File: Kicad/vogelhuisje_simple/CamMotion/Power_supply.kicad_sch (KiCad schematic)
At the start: 11 parts, among them P1 TP4056breakout, P3 TP4056breakout, P4 TP4056breakout, Q1 Q_PMOS_DGS

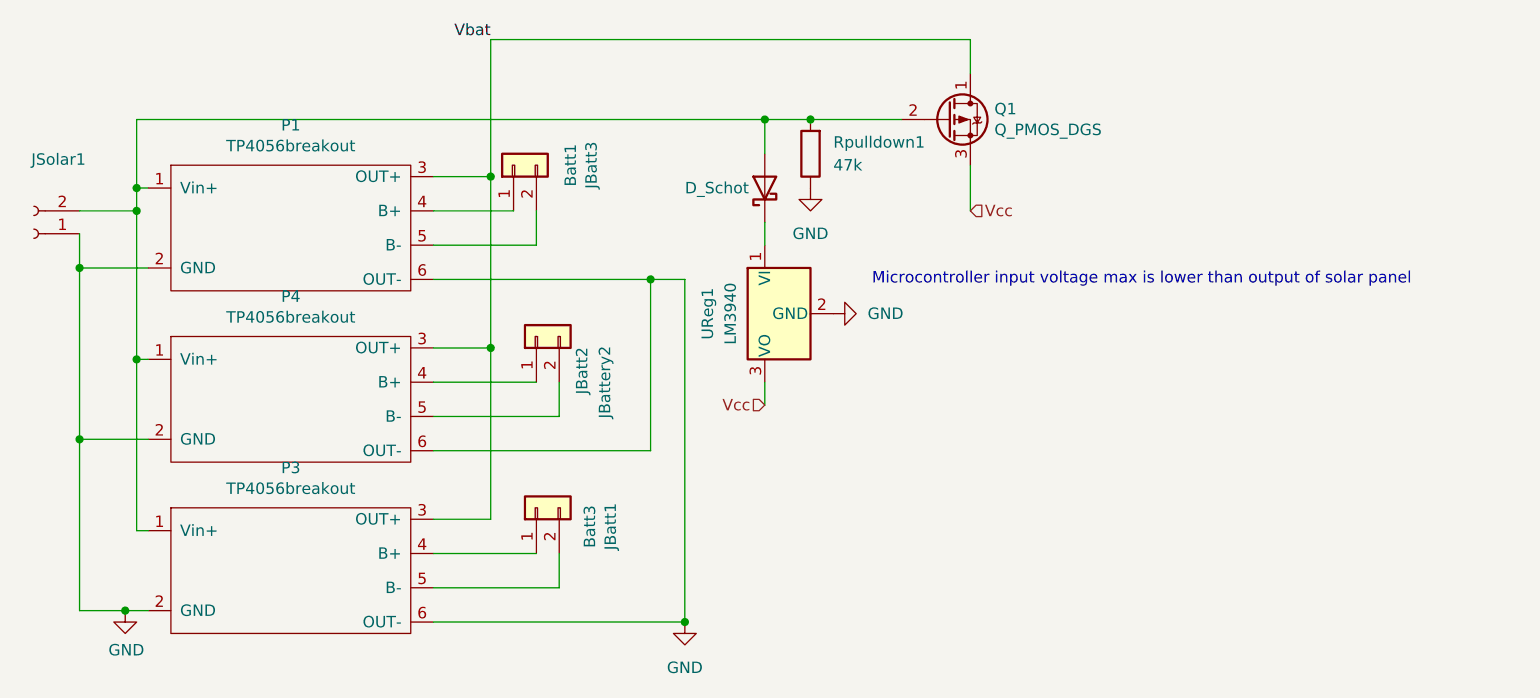
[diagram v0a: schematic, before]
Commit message: Finished PCB
Now more properly routed
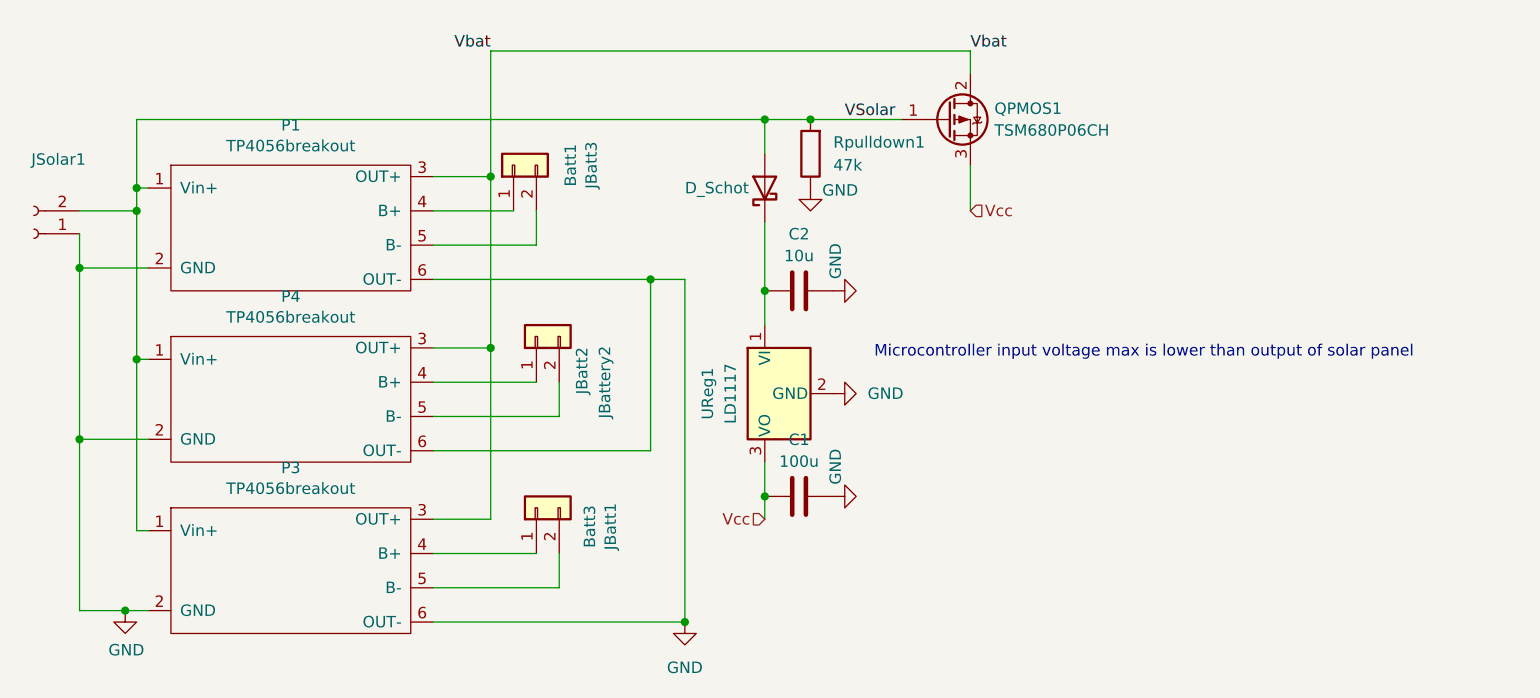
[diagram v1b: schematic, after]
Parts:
- removed Q1: Q_PMOS_DGS, Package_TO_SOT_THT:TO-220-3_Vertical, symbol Device:Q_PMOS_DGS
- added C1: 100u, Capacitor_THT:C_Axial_L5.1mm_D3.1mm_P15.00mm_Horizontal, symbol Device:C
- added C2: 10u, Capacitor_THT:C_Axial_L5.1mm_D3.1mm_P15.00mm_Horizontal, symbol Device:C
- added QPMOS1: TSM680P06CH, Package_TO_SOT_THT:TO-251-3-1EP_Horizontal_TabDown, symbol Device:Q_PMOS_GDS
- UReg1: value LM3940 -> LD1117
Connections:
- net GND: now also C1.2, C2.2
- net Vbat: now also QPMOS1.2 (D)
- net Vcc: now also C1.1, QPMOS1.3 (S)
- net VSolar: now reaches D1.2 (A), JSolar1.2 (Pin_2), P1.1 (Vin+), P3.1 (Vin+), P4.1 (Vin+), Rpulldown1.2
- net VSolar: now also QPMOS1.1 (G)
- net at D1.1 (K), UReg1.1 (VI): now also C2.1
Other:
- moved on the sheet: UReg1
